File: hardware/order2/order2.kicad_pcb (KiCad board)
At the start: 2 copper layers, 377.8 x 228.9 mm, 183 parts, among them IC1 ATMEGA88-A, IC1 ATMEGA88A-A, J1 RJ45, J1 RJ45_8P8C_8FACH, K1 CONN_3, K1 pow_sel, K2 CONN_3, P1 CONN_4, P1 CONN_8, P1 ISP, P1 UART, P10 CONN_10, P11 CONN_8, P2 CONN_4, P2 CONN_6, P2 Shield, P2 UART, P2 so8, P3 CONN_4, P3 CONN_6, P3 i2c_pow, P4 CONN_8, P4 i2c_chain, P5 12Vin, P5 POW, P6 HOHLBUCHSE, P6 TWI, P7 TWI_POW, P7 Vccin, P8 CONN_10, P8 ISP, P9 5Vin, P9 CONN_8, SW1 SW1, SW1 SW_RESET, SW2 SCHALTER_2POL, SW3 SW_RESET, U1 LM7805, U1 ST485, U1 TSIC50XF, U2 HYT271, U2 ST485, U3 ST485, U4 ST485, U5 ST485, U6 ST485, U7 ST485, U8 ST485, U9 ST485, X1 20MHz, m3_loch VAL**

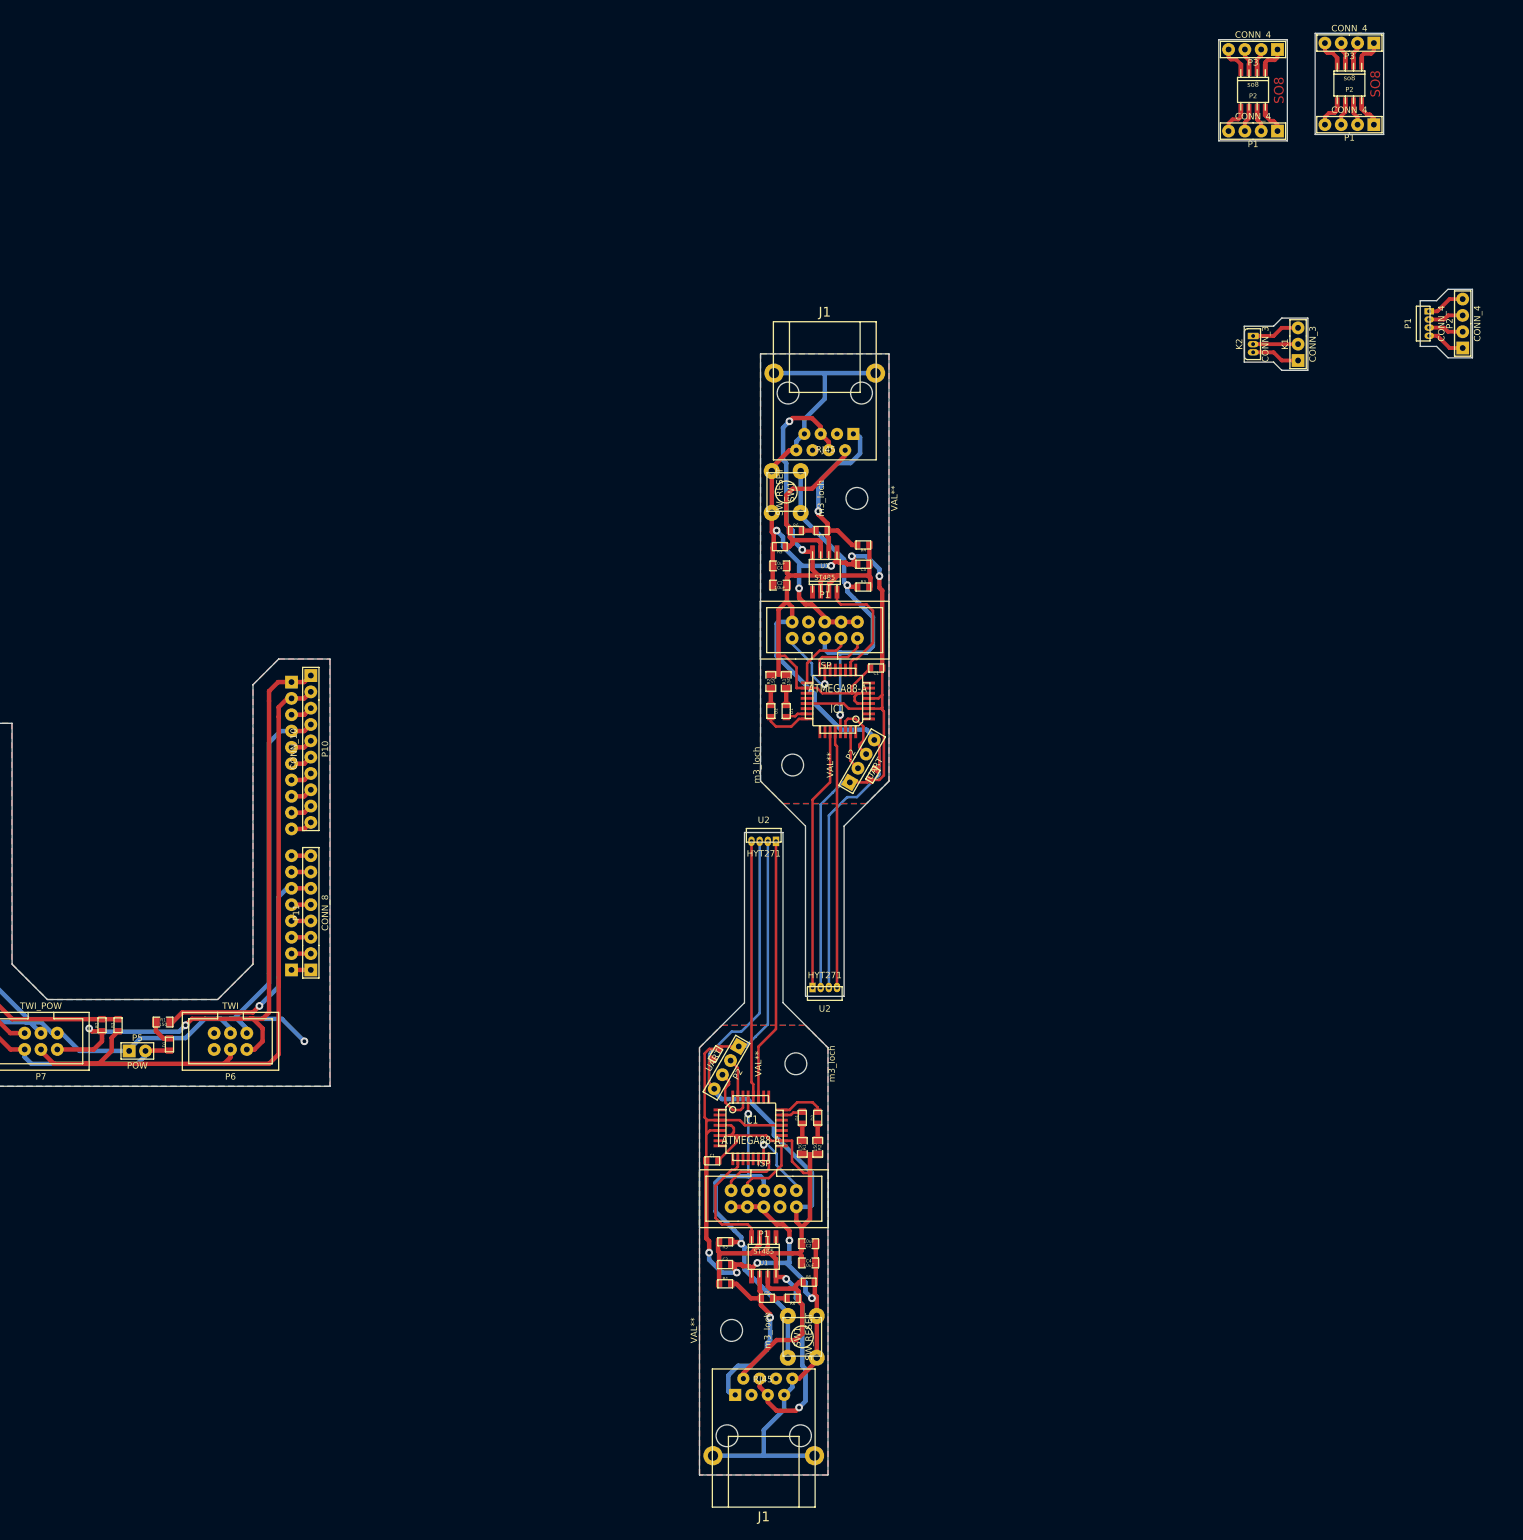
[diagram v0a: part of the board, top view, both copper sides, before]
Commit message: humidity in place
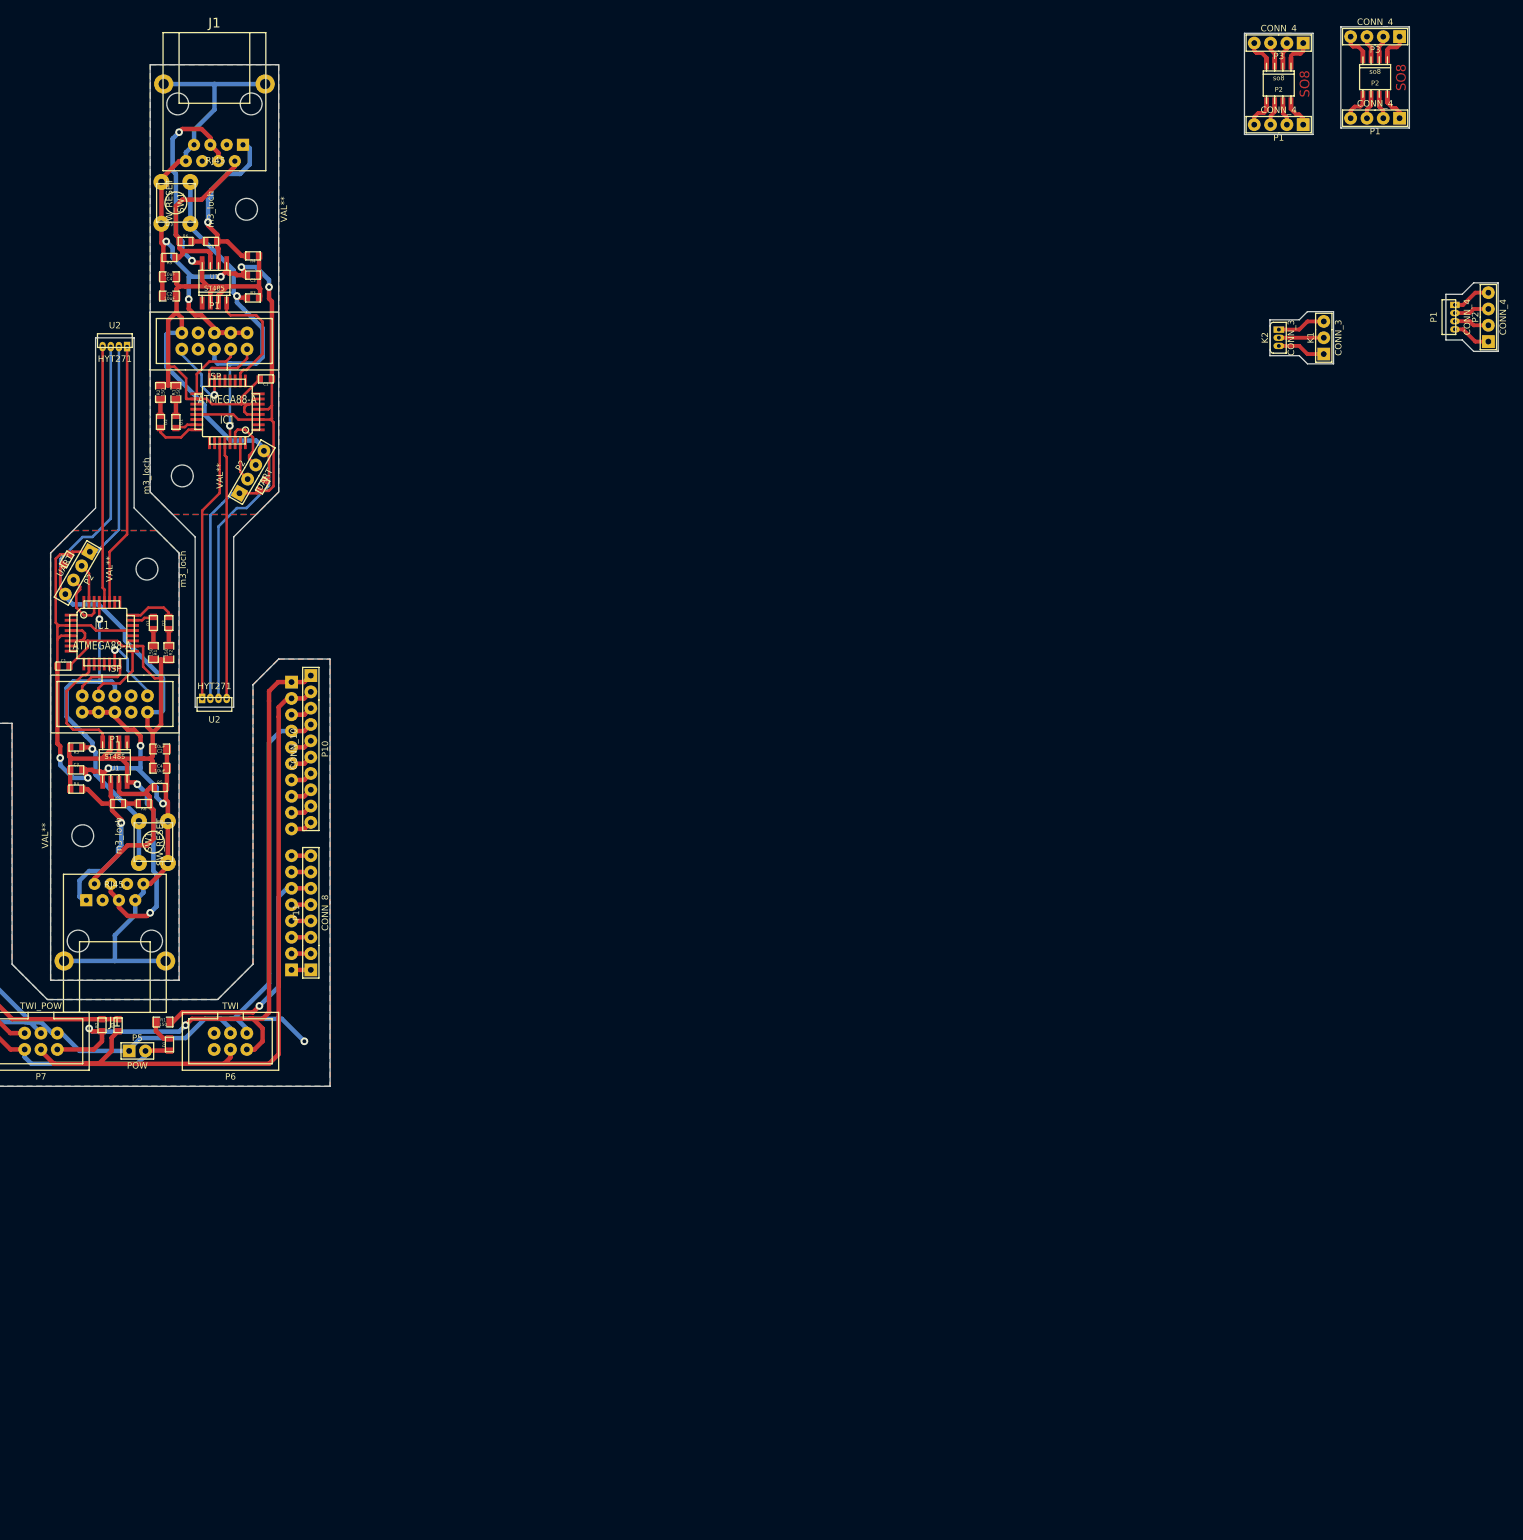
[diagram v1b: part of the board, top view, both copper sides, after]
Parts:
- moved C1 127.0 mm to (178.5, 119.6)
- moved C2 127.0 mm to (193.5, 132.5)
- moved C3 127.0 mm to (180.5, 135.8)
- moved C4 127.0 mm to (193.5, 135.5)
- moved C5 127.0 mm to (187.0, 141.0)
- moved C6 127.0 mm to (179.0, 103.0)
- moved D1 127.0 mm to (192.5, 112.9)
- moved IC1 127.0 mm to (184.5, 114.5)
- moved J1 127.0 mm to (186.5, 153.5)
- moved P1 127.0 mm to (186.5, 125.5)
- moved P2 127.0 mm to (180.7, 105.1)
- moved R1 127.0 mm to (192.5, 117.5)
- moved R3 127.0 mm to (180.5, 132.2)
- moved R4 127.0 mm to (180.5, 138.8)
- moved R5 127.0 mm to (193.5, 138.5)
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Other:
- board size 377.8 x 228.9 mm -> 381.8 x 229.9 mm
